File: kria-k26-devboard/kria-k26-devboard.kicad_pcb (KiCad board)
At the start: 8 copper layers, 121.5 x 89.8 mm, 280 parts, among them IC1 TPS2378DDA, IC2 USB5534B-5000JZX, J1 5-2337992-8, J2 USB4105-GF-A, J3 DC_SOCKET, J4 WE_68715014522, J5 47272-0001, J6 1140084168, M1 XILINX-KRIA-K26, P1 2199119-6, Q1 BSS138DW-7-F, Q2 PJA3441, U1 DP83867CRRGZR, U10 AP62301WU-7, U11 AP62301WU-7, U12 LTC4358CDE, U13 LTC4358CDE, U14 LTC4358CDE, U15 USB3310C-CP, U16 TPD4E05U06QDQARQ1, U17 TPD4E05U06QDQARQ1, U18 GSB3112311HR, U19 TPD4E05U06QDQARQ1, U2 MAX5984AETI+T, U20 TPD4E05U06QDQARQ1, U21 GSB3112311HR, U22 PI4MSD5V9540BUEX, U23 FT4232HPQ, U24 SN74AVC4T245PWR, U25 FIN1019MTC, U26 TPD4E05U06QDQARQ1, U27 NVT4858HKZ, U28 TPS2116DRLR, U3 AP62301WU-7, U4 AP62301WU-7, U5 AP62301WU-7, U6 AP62301WU-7, U7 AP62301WU-7, U8 RPX-4.0-R, U9 AP62301WU-7, Y1 ABM8G-25.000MHZ-18-D2Y-T

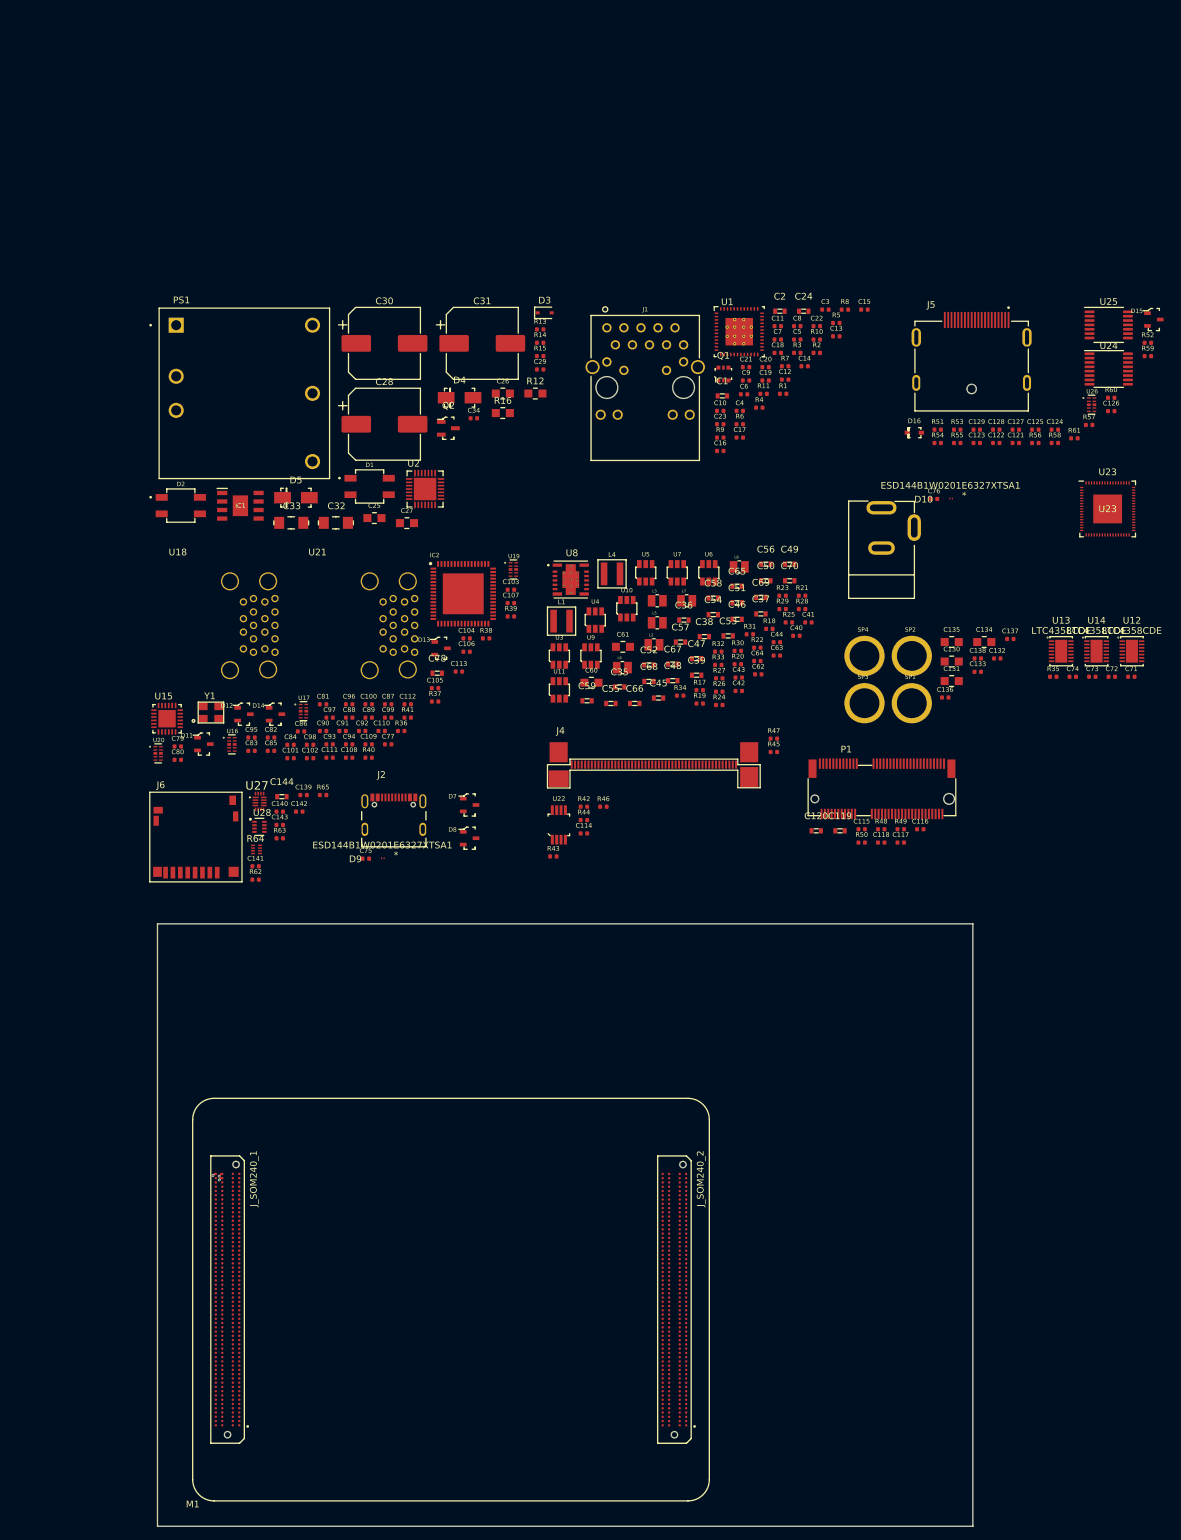
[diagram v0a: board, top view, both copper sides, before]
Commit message: Progress on Debug sheet
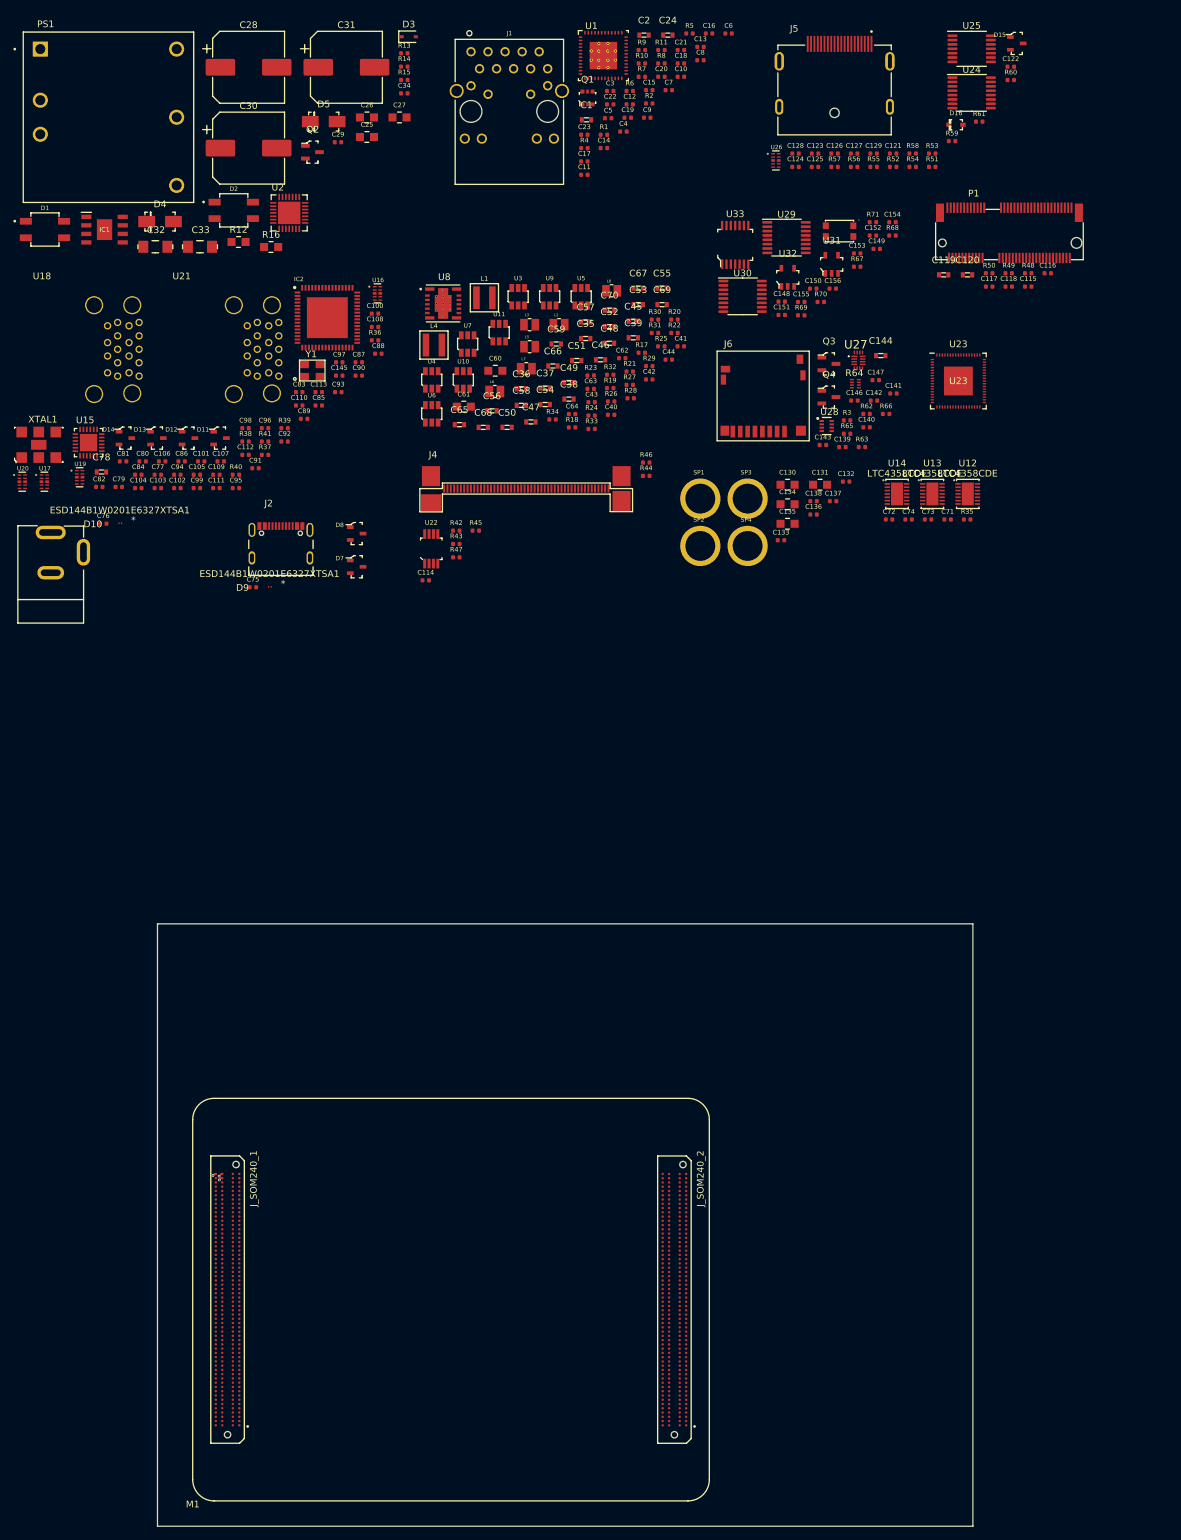
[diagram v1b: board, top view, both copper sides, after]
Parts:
- added C145: C_100n_0402, antmicro-footprints:0402-cap, F.Cu at (103.3, -34.5)
- added C146: C_470n_0402, antmicro-footprints:0402-cap, F.Cu at (180.1, -30.8)
- added C147: C_470n_0402, antmicro-footprints:0402-cap, F.Cu at (183.2, -33.9)
- added C148: C_100n_0402, antmicro-footprints:0402-cap, F.Cu at (169.2, -45.6)
- added C149: C_100n_0402, antmicro-footprints:0402-cap, F.Cu at (183.4, -53.4)
- added C150: C_47n_0402, antmicro-footprints:0402-cap, F.Cu at (173.9, -47.5)
- added C151: C_47n_0402, antmicro-footprints:0402-cap, F.Cu at (169.2, -43.6)
- added C152: C_100n_0402, antmicro-footprints:0402-cap, F.Cu at (182.8, -55.4)
- added C153: C_100n_0402, antmicro-footprints:0402-cap, F.Cu at (180.5, -52.8)
- added C154: C_100n_0402, antmicro-footprints:0402-cap, F.Cu at (185.7, -57.4)
- added C155: C_100n_0402, antmicro-footprints:0402-cap, F.Cu at (172.1, -45.5)
- added C156: C_100n_0402, antmicro-footprints:0402-cap, F.Cu at (176.8, -47.5)
- added Q3: BSS123, antmicro-footprints:SOT-23-3, F.Cu at (176.2, -36.3)
- added Q4: AO3401A, antmicro-footprints:SOT-23-3, F.Cu at (176.2, -31.3)
- added R66: R_1k_0402, antmicro-footprints:0402-res, F.Cu at (184.8, -28.8)
- added R67: R_10k_0402, antmicro-footprints:0402-res, F.Cu at (180.5, -50.8)
- added R68: R_10k_0402, antmicro-footprints:0402-res, F.Cu at (185.7, -55.4)
- added R69: R_10k_0402, antmicro-footprints:0402-res, F.Cu at (172.1, -43.5)
- added R70: R_10k_0402, antmicro-footprints:0402-res, F.Cu at (175.0, -45.5)
- added R71: R_10k_0402, antmicro-footprints:0402-res, F.Cu at (182.8, -57.4)
- added S1: KMR2, antmicro-footprints:SW_SPST_4.2x2.8, F.Cu at (177.8, -56.1)
- added U29: SN74AVC4T245PWR, Package_SO:TSSOP-16_4.4x5mm_P0.65mm, F.Cu at (169.9, -55.1)
- added U30: SN74AVC4T245PWR, Package_SO:TSSOP-16_4.4x5mm_P0.65mm, F.Cu at (163.4, -46.4)
- added U31: TPS3840PH30DBVR, antmicro-footprints:SOT-23-5, F.Cu at (176.7, -51.1)
- added U32: TPS3840PH30DBVR, antmicro-footprints:SOT-23-5, F.Cu at (170.1, -49.2)
- added U33: 74LV07ATPWJ, antmicro-footprints:TSSOP-14_W4.4mm, F.Cu at (162.3, -54.0)
- added XTAL1: SIT1602BC-13-18E-24.000000G, antmicro-footprints:SiTIME_SMD-6-1EP, F.Cu at (58.5, -24.2)
- moved D10 123.9 mm to (70.6, -12.5)
- moved C76 123.9 mm to (68.1, -12.5)
- moved J3 123.9 mm to (60.3, 2.53)
- moved C141 118.3 mm to (185.9, -31.9)
- moved R62 114.5 mm to (181.9, -28.8)
- moved R64 113.1 mm to (180.2, -33.3)
- moved C144 110.8 mm to (184.0, -37.5)
- moved U27 110.8 mm to (180.7, -36.8)
- moved J6 107.1 mm to (166.5, -31.5)
- moved C142 105.3 mm to (183.0, -30.8)
- moved C140 104.5 mm to (181.9, -26.8)
- moved R63 104.5 mm to (181.2, -23.9)
- moved U28 103.5 mm to (175.9, -27.0)
- moved C143 98.8 mm to (175.4, -24.2)
- moved C139 95.6 mm to (178.3, -23.9)
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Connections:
- IC2 pad 50: Net-(IC2-Pad50) -> /Reset logic/USB_HUB_RESET
- J4 pad 32: Net-(J4-Pad32) -> /Camera interfaces/CAM0_PWDN
- J4 pad 33: Net-(J4-Pad33) -> /Camera interfaces/CAM0_RST
- J4 pad 34: Net-(J4-Pad34) -> /Camera interfaces/CAM1_PWDN
- J_SOM240_1 pad A15: /Xilinx K26 SOM/HDA09 -> /Reset logic/HDA09
- J_SOM240_1 pad A36: /Xilinx K26 SOM/MIO43 -> /Reset logic/MIO43
- J_SOM240_1 pad B13: /Xilinx K26 SOM/VCCO_HDA -> PL_3V3
- J_SOM240_1 pad B14: /Xilinx K26 SOM/VCCO_HDA -> PL_3V3
- J_SOM240_1 pad B17: /Xilinx K26 SOM/HDA04 -> /Reset logic/HDA04
- J_SOM240_1 pad B32: /Xilinx K26 SOM/MIO38 -> /Reset logic/MIO38
- J_SOM240_1 pad D01: PL_3V3 -> PL_1V2
- J_SOM240_1 pad D02: PL_3V3 -> PL_1V2
- J_SOM240_1 pad D18: /Xilinx K26 SOM/HDA02 -> /Reset logic/HDA02
- J_SOM240_1 pad D32: /Xilinx K26 SOM/MIO44 -> /Reset logic/MIO44
- R3 pad 1: PS_1V8 -> PS_3V3
- R3 pad 2: /Ethernet/ETH_RESET -> Net-(C146-Pad2)
- U15 pad 14: Net-(U15-Pad14) -> PS_1V8
- U15 pad 15: Net-(U15-Pad14) -> PS_1V8
- U15 pad 22: Net-(U15-Pad22) -> /Reset logic/USB_PHY_RESET
